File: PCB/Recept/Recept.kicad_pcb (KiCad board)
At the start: 4 copper layers, 69 x 120.5 mm, 132 parts, among them J1 Conn_01x02_Pin, J2 Conn_02x03_Counter_Clockwise, J4 Conn_02x04_Counter_Clockwise, J5 Conn_02x02_Counter_Clockwise, SW1 SW_Push, SW15 DSIC03LSGET, SW16 SW_Push, SW18 K3-1204D-L, U1 RP2040, U2 ABM8-272-T3_C20625731, U24 TPS630701RNMT, U25 BQ21088YBGR, U27 LD1117S33TR_SOT223, U28 CAT4104, U29 MT3608, U30 SMA_Conn, U31 LD1117S18TR_SOT223, U4 W25Q16JVZPIQ, X3 X322527MSB4SI

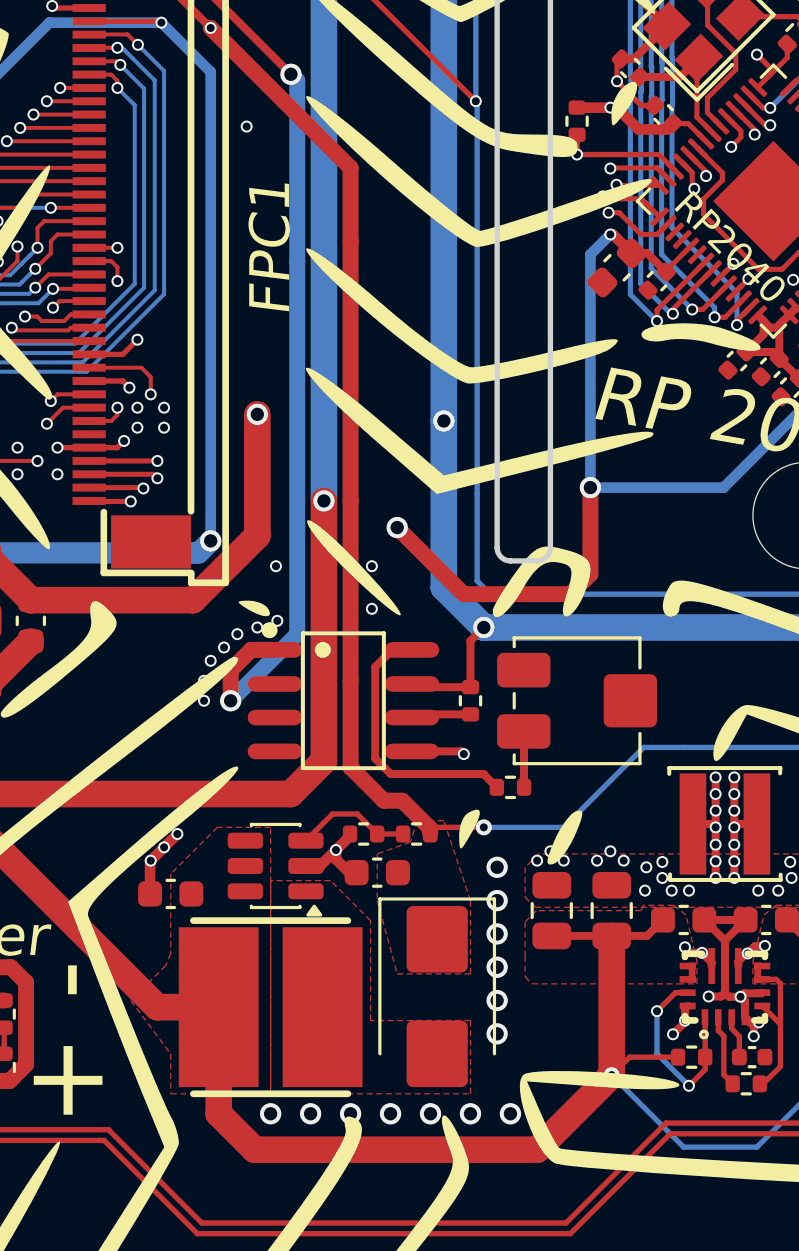
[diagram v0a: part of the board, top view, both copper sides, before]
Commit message: Update
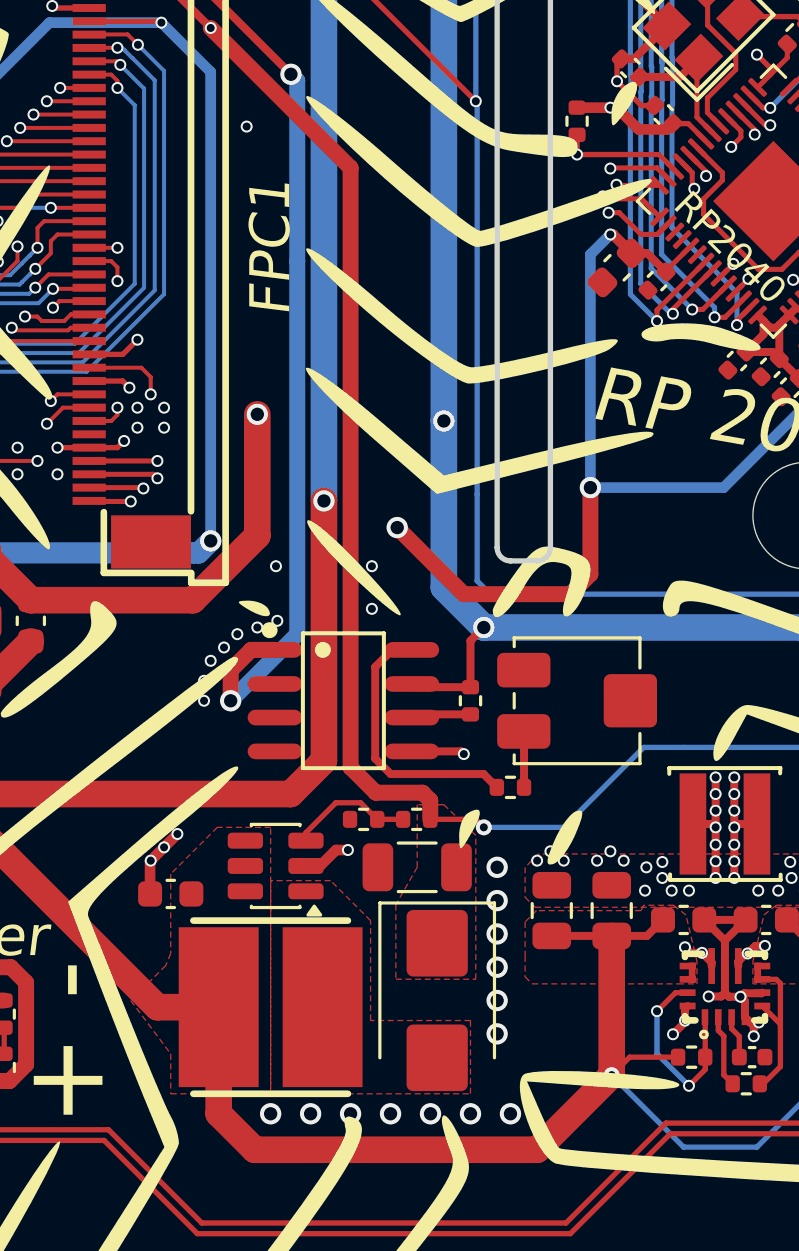
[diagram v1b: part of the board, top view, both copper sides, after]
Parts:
- C98: footprint Capacitor_SMD:C_0603_1608Metric -> Capacitor_SMD:C_1206_3216Metric
- moved C98 1.51 mm to (120.0, 95.0)
- moved R105 0.55 mm to (120.0, 93.2)
- moved R95 0.55 mm to (118.0, 93.2)
- moved D10 0.15 mm to (120.8, 100.0)
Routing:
- net GND: track 152.3 -> 150.6 mm
